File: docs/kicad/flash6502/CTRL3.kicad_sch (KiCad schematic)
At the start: 16 parts

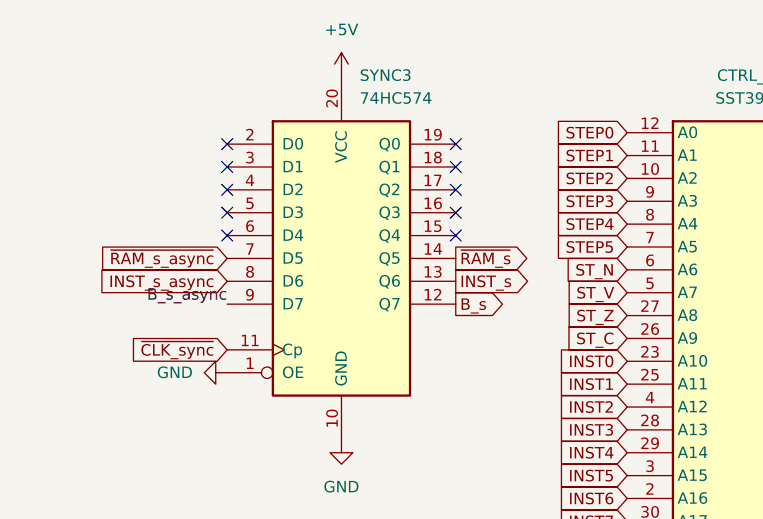
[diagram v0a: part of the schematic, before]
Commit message: ok, docs
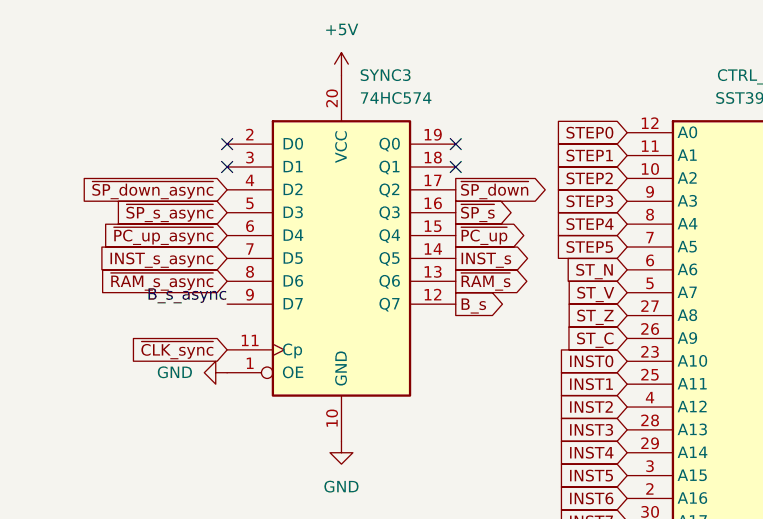
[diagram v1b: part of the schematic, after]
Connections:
- net INST_s: now also SYNC3.14 (Q5); no longer SYNC3.13 (Q6)
- net INST_s_async: now also SYNC3.7 (D5); no longer SYNC3.8 (D6)
- net ~{RAM_s_async}: now also SYNC3.8 (D6); no longer SYNC3.7 (D5)
- net ~{RAM_s}: now also SYNC3.13 (Q6); no longer SYNC3.14 (Q5)
- net ~{PC_up}: now reaches SYNC3.15 (Q4)
- net ~{SP_s}: now reaches SYNC3.16 (Q3)
- net ~{SP_down}: now reaches SYNC3.17 (Q2)
- net ~{SP_down_async}: now reaches SYNC3.4 (D2)
- net ~{SP_s_async}: now reaches SYNC3.5 (D3)
- net ~{PC_up_async}: now reaches SYNC3.6 (D4)
- no-connect marks 14 -> 8
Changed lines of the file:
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@@
   (no_connect (at 214.63 41.91))
   (no_connect (at 214.63 44.45))
-  (no_connect (at 64.77 41.91))
   (no_connect (at 64.77 36.83))
-  (no_connect (at 39.37 46.99))
   (no_connect (at 39.37 36.83))
   (no_connect (at 83.82 81.28))
-  (no_connect (at 39.37 41.91))
   (no_connect (at 64.77 39.37))
-  (no_connect (at 64.77 44.45))
   (no_connect (at 214.63 49.53))
-  (no_connect (at 39.37 44.45))
   (no_connect (at 39.37 39.37))
-  (no_connect (at 64.77 46.99))
   (wire (pts (xy 170.18 49.53) (xy 170.18 54.61))
     (stroke (width 0) (type default) (color 0 0 0 0))
@@
     )
   )
-  (global_label "INST_s" (shape output) (at 64.77 52.07 0) (fields_autoplaced)
-    (effects (font (size 1.27 1.27)) (justify left))
-    (property "Intersheet References" "${INTERSHEET_REFS}" (id 0) (at 73.2912 51.9906 0)
+  (global_label "~{SP_s}" (shape output) (at 64.77 44.45 0) (fields_autoplaced)
+    (effects (font (size 1.27 1.27)) (justify left))
+    (property "Intersheet References" "${INTERSHEET_REFS}" (id 0) (at 71.6583 44.3706 0)
       (effects (font (size 1.27 1.27)) (justify left) hide)
     )
@@
     )
   )
-  (global_label "~{RAM_s}" (shape output) (at 64.77 49.53 0) (fields_autoplaced)
-    (effects (font (size 1.27 1.27)) (justify left))
-    (property "Intersheet References" "${INTERSHEET_REFS}" (id 0) (at 72.9888 49.4506 0)
-      (effects (font (size 1.27 1.27)) (justify left) hide)
-    )
-  )
   (global_label "ALU_op2" (shape output) (at 114.3 50.8 0) (fields_autoplaced)
     (effects (font (size 1.27 1.27)) (justify left))
@@
     )
   )
+  (global_label "~{SP_down_async}" (shape input) (at 39.37 41.91 180) (fields_autoplaced)
+    (effects (font (size 1.27 1.27)) (justify right))
+    (property "Intersheet References" "${INTERSHEET_REFS}" (id 0) (at 22.3821 41.8306 0)
+      (effects (font (size 1.27 1.27)) (justify right) hide)
+    )
+  )
   (global_label "~{CLK_async}" (shape input) (at 189.23 57.15 180) (fields_autoplaced)
     (effects (font (size 1.27 1.27)) (justify right))
@@
     )
   )
+  (global_label "INST_s_async" (shape input) (at 39.37 49.53 180) (fields_autoplaced)
+    (effects (font (size 1.27 1.27)) (justify right))
+    (property "Intersheet References" "${INTERSHEET_REFS}" (id 0) (at 24.4988 49.4506 0)
+      (effects (font (size 1.27 1.27)) (justify right) hide)
+    )
+  )
+  (global_label "~{RAM_s}" (shape output) (at 64.77 52.07 0) (fields_autoplaced)
+    (effects (font (size 1.27 1.27)) (justify left))
+    (property "Intersheet References" "${INTERSHEET_REFS}" (id 0) (at 72.9888 51.9906 0)
+      (effects (font (size 1.27 1.27)) (justify left) hide)
+    )
+  )
   (global_label "ST_V" (shape input) (at 83.82 53.34 180) (fields_autoplaced)
     (effects (font (size 1.27 1.27)) (justify right))
@@
     )
   )
+  (global_label "INST_s" (shape output) (at 64.77 49.53 0) (fields_autoplaced)
+    (effects (font (size 1.27 1.27)) (justify left))
+    (property "Intersheet References" "${INTERSHEET_REFS}" (id 0) (at 73.2912 49.4506 0)
+      (effects (font (size 1.27 1.27)) (justify left) hide)
+    )
+  )
   (global_label "STEP5" (shape input) (at 257.81 87.63 0) (fields_autoplaced)
     (effects (font (size 1.27 1.27)) (justify left))
@@
     )
   )
-  (global_label "INST_s_async" (shape input) (at 39.37 52.07 180) (fields_autoplaced)
-    (effects (font (size 1.27 1.27)) (justify right))
-    (property "Intersheet References" "${INTERSHEET_REFS}" (id 0) (at 24.4988 51.9906 0)
+  (global_label "~{PC_up}" (shape output) (at 64.77 46.99 0) (fields_autoplaced)
+    (effects (font (size 1.27 1.27)) (justify left))
+    (property "Intersheet References" "${INTERSHEET_REFS}" (id 0) (at 72.9888 46.9106 0)
+      (effects (font (size 1.27 1.27)) (justify left) hide)
+    )
+  )
+  (global_label "~{PC_up_async}" (shape input) (at 39.37 46.99 180) (fields_autoplaced)
+    (effects (font (size 1.27 1.27)) (justify right))
+    (property "Intersheet References" "${INTERSHEET_REFS}" (id 0) (at 24.8012 46.9106 0)
+      (effects (font (size 1.27 1.27)) (justify right) hide)
+    )
+  )
+  (global_label "~{SP_s_async}" (shape input) (at 39.37 44.45 180) (fields_autoplaced)
+    (effects (font (size 1.27 1.27)) (justify right))
+    (property "Intersheet References" "${INTERSHEET_REFS}" (id 0) (at 26.1317 44.3706 0)
       (effects (font (size 1.27 1.27)) (justify right) hide)
     )
@@
     )
   )
-  (global_label "~{RAM_s_async}" (shape input) (at 39.37 49.53 180) (fields_autoplaced)
-    (effects (font (size 1.27 1.27)) (justify right))
-    (property "Intersheet References" "${INTERSHEET_REFS}" (id 0) (at 24.8012 49.4506 0)
-      (effects (font (size 1.27 1.27)) (justify right) hide)
+  (global_label "~{SP_down}" (shape output) (at 64.77 41.91 0) (fields_autoplaced)
+    (effects (font (size 1.27 1.27)) (justify left))
+    (property "Intersheet References" "${INTERSHEET_REFS}" (id 0) (at 75.4079 41.8306 0)
+      (effects (font (size 1.27 1.27)) (justify left) hide)
     )
   )
@@
     )
   )
+  (global_label "~{RAM_s_async}" (shape input) (at 39.37 52.07 180) (fields_autoplaced)
+    (effects (font (size 1.27 1.27)) (justify right))
+    (property "Intersheet References" "${INTERSHEET_REFS}" (id 0) (at 24.8012 51.9906 0)
+      (effects (font (size 1.27 1.27)) (justify right) hide)
+    )
+  )
